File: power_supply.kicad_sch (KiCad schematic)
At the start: 18 parts, among them J1 Разъём к автомобилю 2x16 (32 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, U6 MC78M05CDTG, U7 AMS1117-3.3

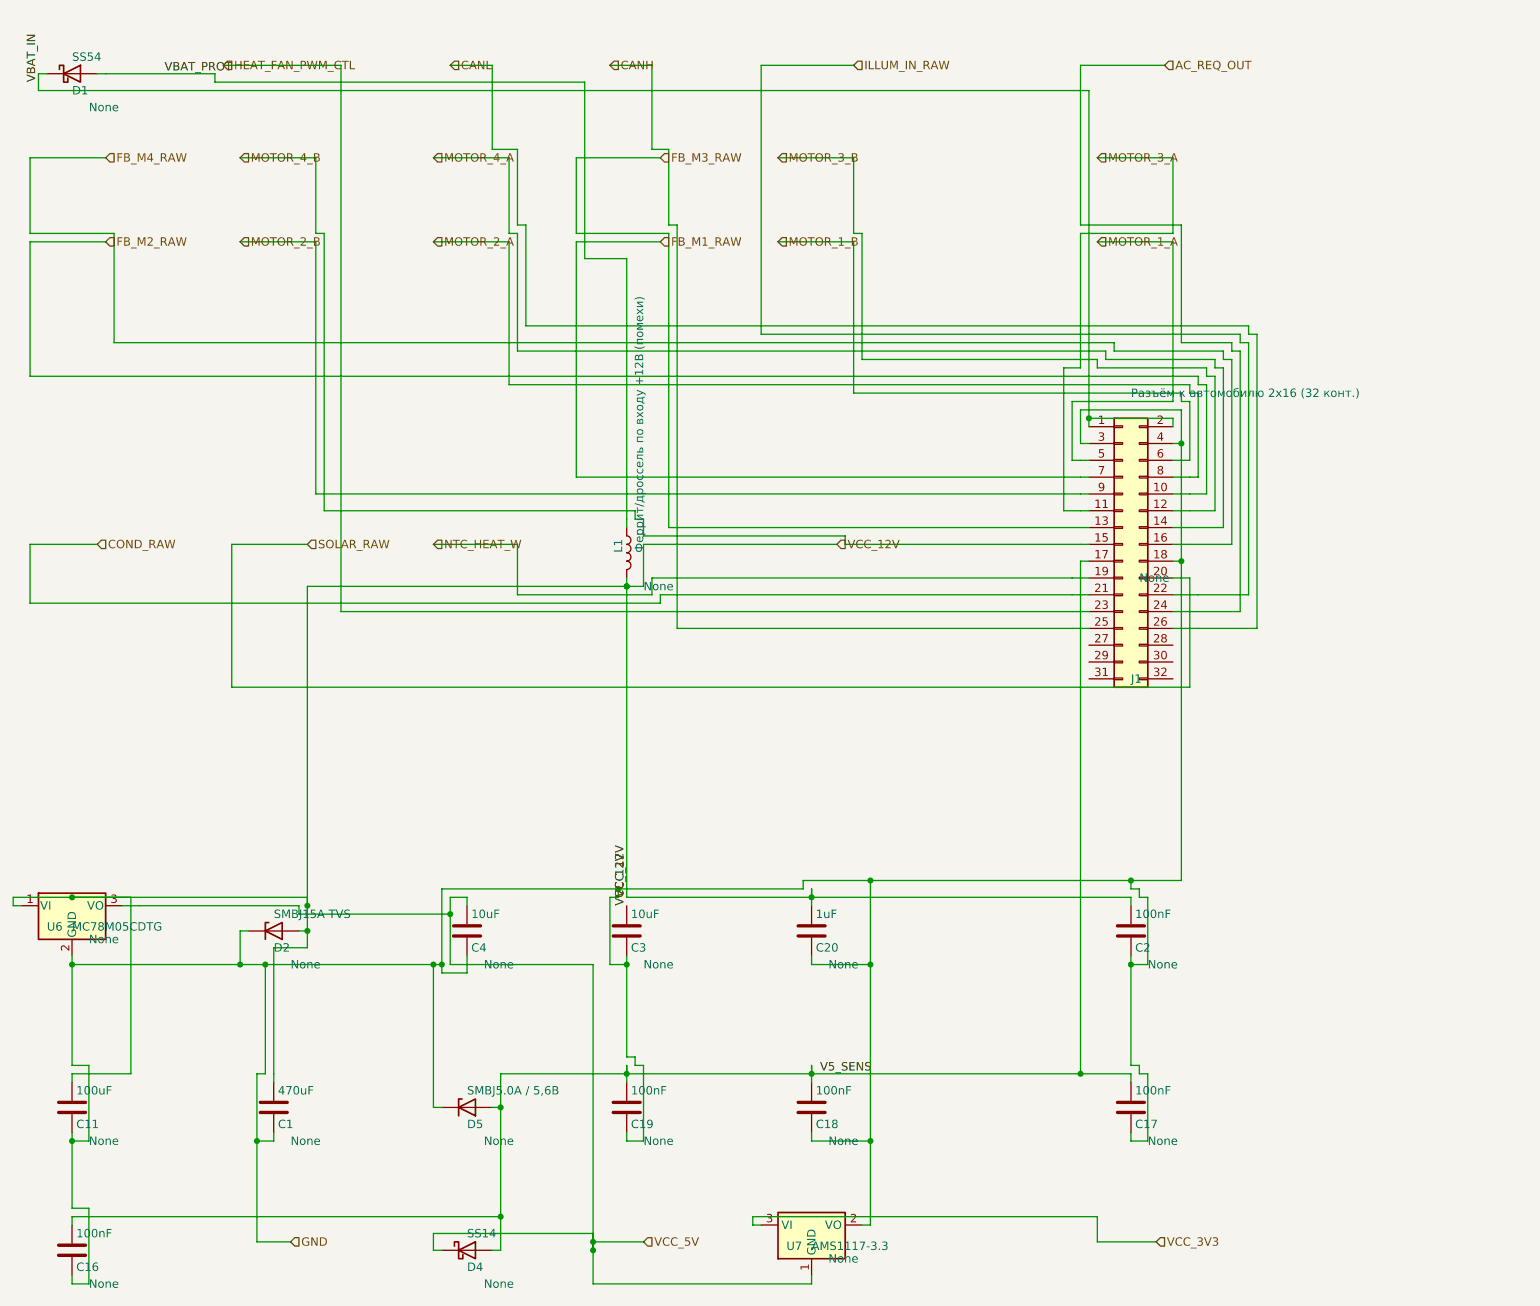
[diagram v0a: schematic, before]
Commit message: all unit test pass
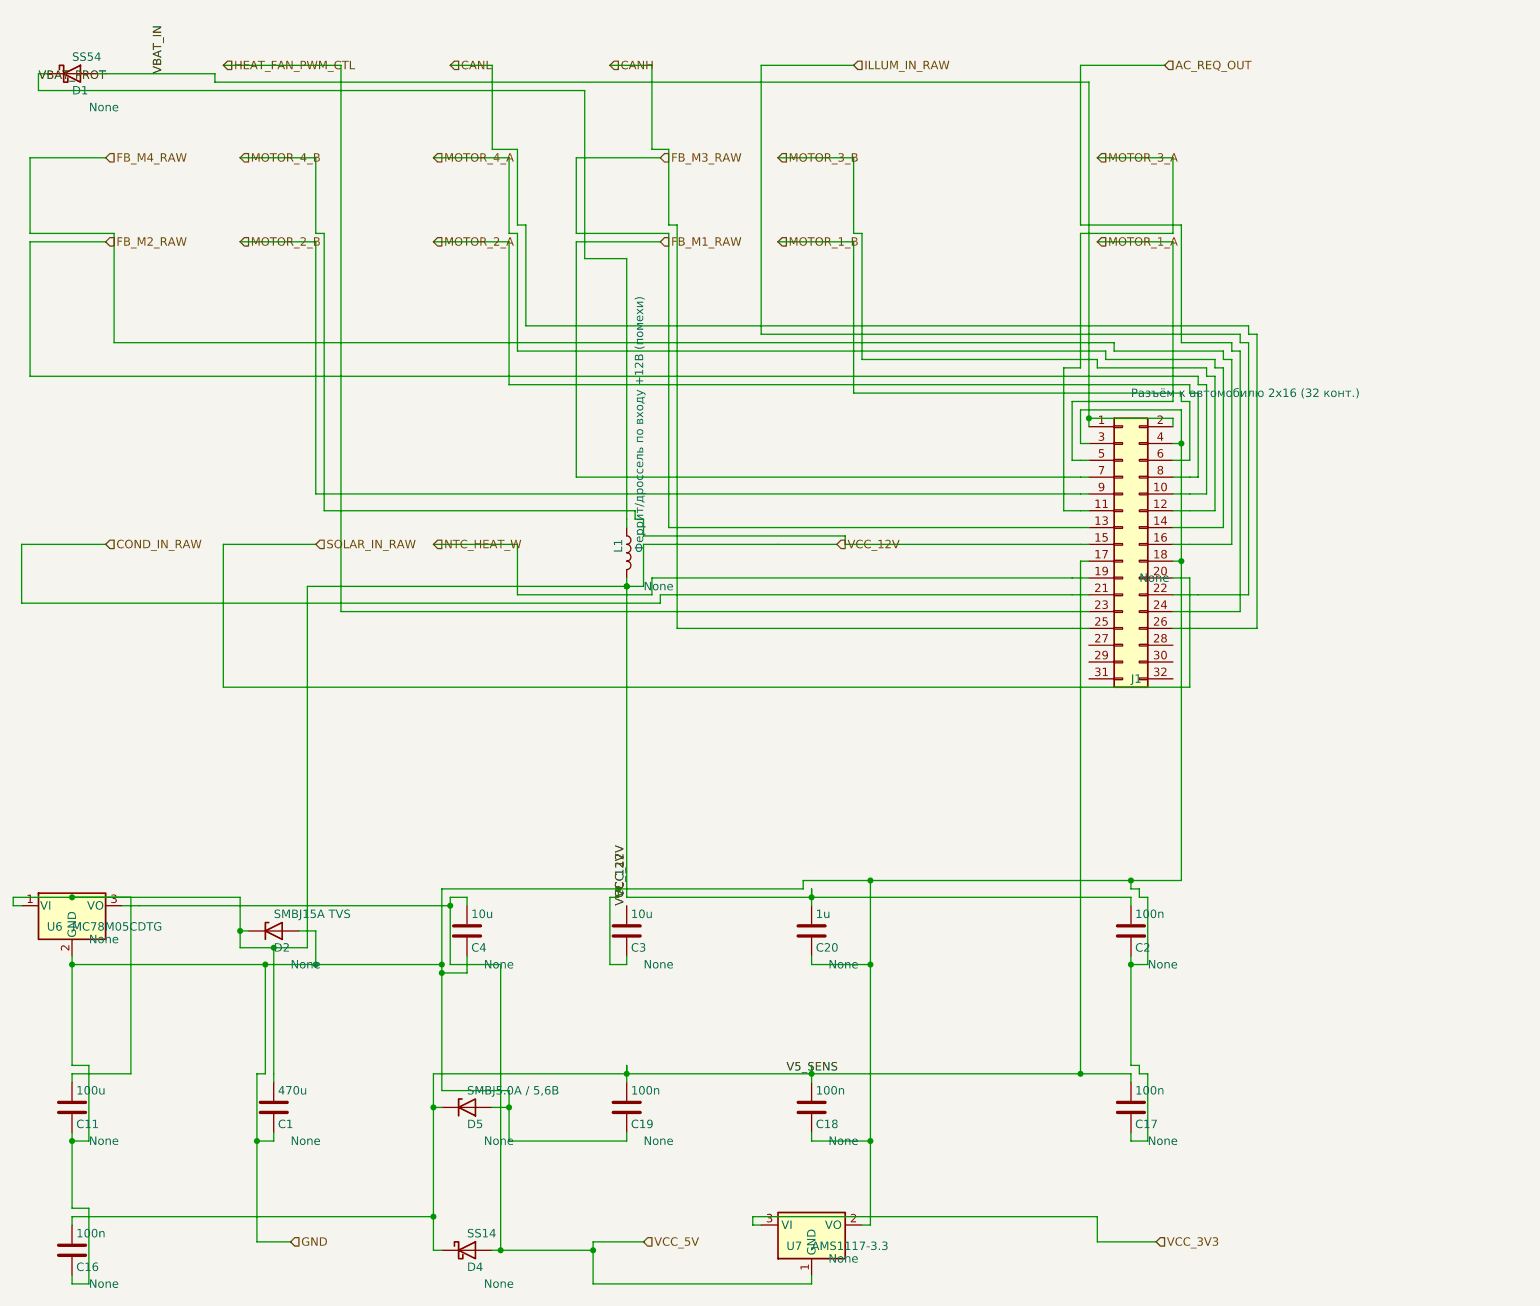
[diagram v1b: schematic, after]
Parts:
- C1: value 470uF -> 470u
- C11: value 100uF -> 100u
- C16, C17, C18, C19, C2: value 100nF -> 100n
- C20: value 1uF -> 1u
- C3, C4: value 10uF -> 10u
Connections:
- net GND: now also D2.2 (A), D5.2 (A); no longer D2.1 (K), D5.1 (K)
- net V5_SENS: now also D4.1 (K), D5.1 (K); no longer D4.2 (A), D5.2 (A)
- net VBAT_IN: now also D1.2 (A); no longer D1.1 (K)
- net VBAT_PROT: now also D1.1 (K); no longer D1.2 (A)
- net VCC_12V: now also D2.1 (K); no longer D2.2 (A)
- net VCC_5V: now also D4.2 (A); no longer D4.1 (K)
- net COND_RAW renamed COND_IN_RAW
- net SOLAR_RAW renamed SOLAR_IN_RAW
